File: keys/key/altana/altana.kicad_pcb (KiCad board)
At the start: 2 copper layers, 17.8 x 17.8 mm, 3 parts, among them SW1 SW_PUSH

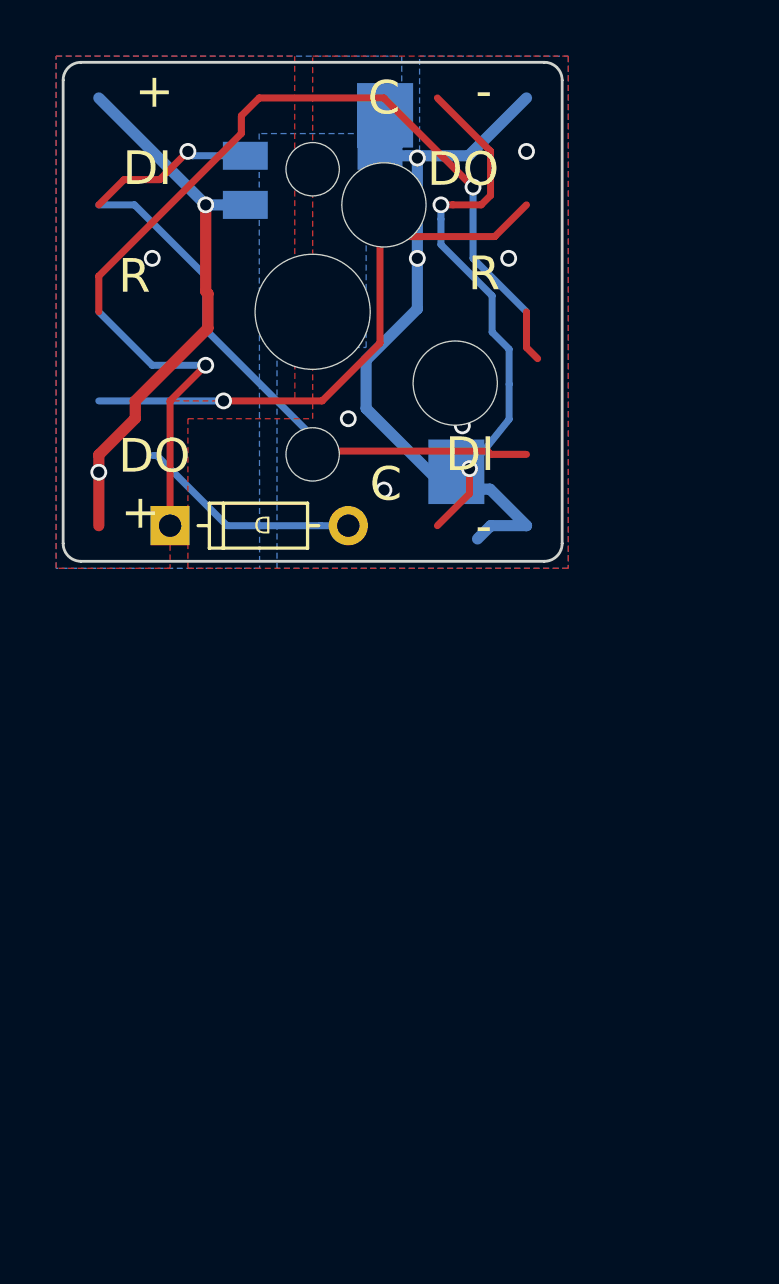
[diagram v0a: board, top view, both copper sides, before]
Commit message: Update
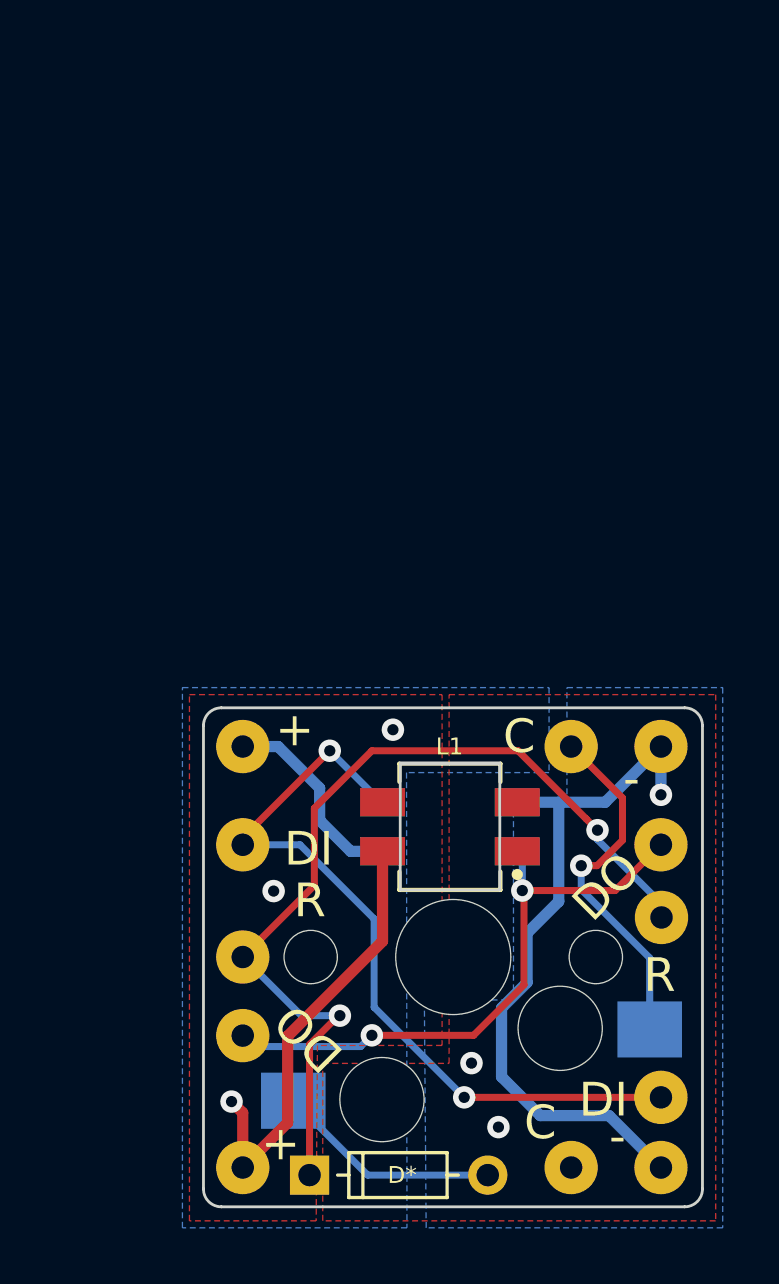
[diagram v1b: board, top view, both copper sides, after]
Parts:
- removed D: D, footprint:diode
- added D1: D, footprint:diode, F.Cu at (153.1, 136.2)
- added J1: (+), kbd:wirepad-h0.8mm-d1.8mm, F.Cu at (150.8, 121.0)
- added J10: R, kbd:wirepad-h0.8mm-d1.8mm, F.Cu at (165.7, 127.0)
- added J11: DI, kbd:wirepad-h0.8mm-d1.8mm, F.Cu at (165.7, 133.5)
- added J12: DO, kbd:wirepad-h0.8mm-d1.8mm, F.Cu at (165.7, 124.5)
- added J2: (-), kbd:wirepad-h0.8mm-d1.8mm, F.Cu at (165.7, 121.0)
- added J3: C, kbd:wirepad-h0.8mm-d1.8mm, F.Cu at (162.5, 136.0)
- added J4: R, kbd:wirepad-h0.8mm-d1.8mm, F.Cu at (150.8, 128.5)
- added J5: DI, kbd:wirepad-h0.8mm-d1.8mm, F.Cu at (150.8, 124.5)
- added J6: DO, kbd:wirepad-h0.8mm-d1.8mm, F.Cu at (150.8, 131.3)
- added J7: (+), kbd:wirepad-h0.8mm-d1.8mm, F.Cu at (150.8, 136.0)
- added J8: (-), kbd:wirepad-h0.8mm-d1.8mm, F.Cu at (165.7, 136.0)
- added J9: C, kbd:wirepad-h0.8mm-d1.8mm, F.Cu at (162.5, 121.0)
- L1: moved to F.Cu
- SW1: value SW_PUSH -> SW_Push
- moved L1 23.5 mm to (158.1, 123.8)
- moved SW1 23.5 mm to (158.3, 128.5), turned to 180 degrees
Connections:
- L1 pad 1: Net-(L1-Pad1) -> /key/LED_DO
- L1 pad 3: Net-(L1-Pad3) -> /key/LED_DI
- SW1 pad 1: /COL0 -> /key/COL_N
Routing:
- net /key/ROW_N: track 0.00 -> 33.0 mm, vias 0 -> 2
- net /key/LED_DI: track 0.00 -> 27.7 mm, vias 0 -> 2
- net GND: track 49.7 -> 25.2 mm, vias 7 -> 3
- net Net-(L1-Pad1): track 21.5 -> 0.00 mm, vias 2 -> 0
- net /key/LED_DO: track 0.00 -> 21.3 mm, vias 0 -> 2
- net (no net): track 20.0 -> 0.00 mm, vias 2 -> 0
- net /COL0: track 19.6 -> 0.00 mm, vias 2 -> 0
- net /key/COL_N: track 0.00 -> 12.8 mm, vias 0 -> 1
- net /ROW0: track 12.7 -> 0.00 mm, vias 1 -> 0
- net Net-(L1-Pad3): track 6.07 -> 0.00 mm, vias 1 -> 0
- net VCC: track 19.9 -> 23.2 mm
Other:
- outline, holes or cut-outs redrawn
